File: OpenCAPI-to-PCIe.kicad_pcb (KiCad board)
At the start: 4 copper layers, 51.3 x 31.9 mm, 9 parts, among them J1 OpenCAPI_AAC_Host, J2 Conn_01x06, J3 Bus_PCI_Express_x8

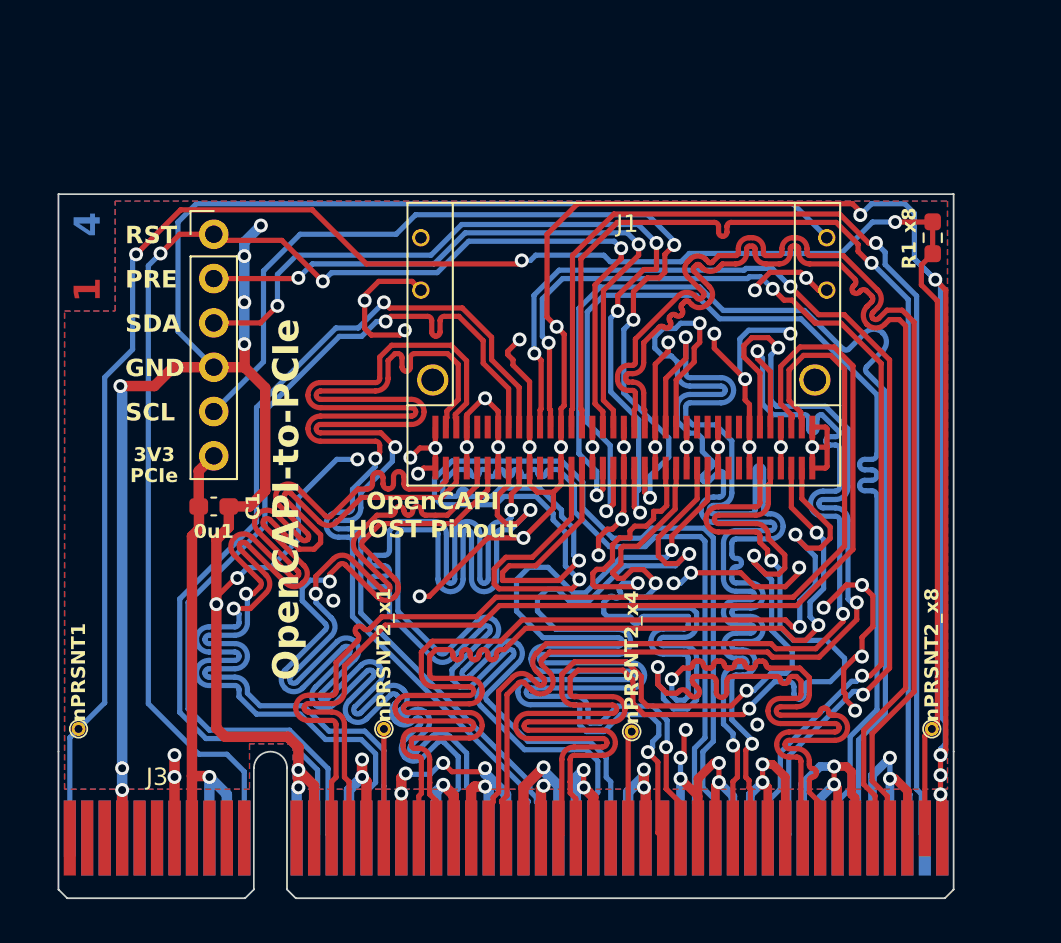
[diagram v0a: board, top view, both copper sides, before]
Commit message: Third Revision
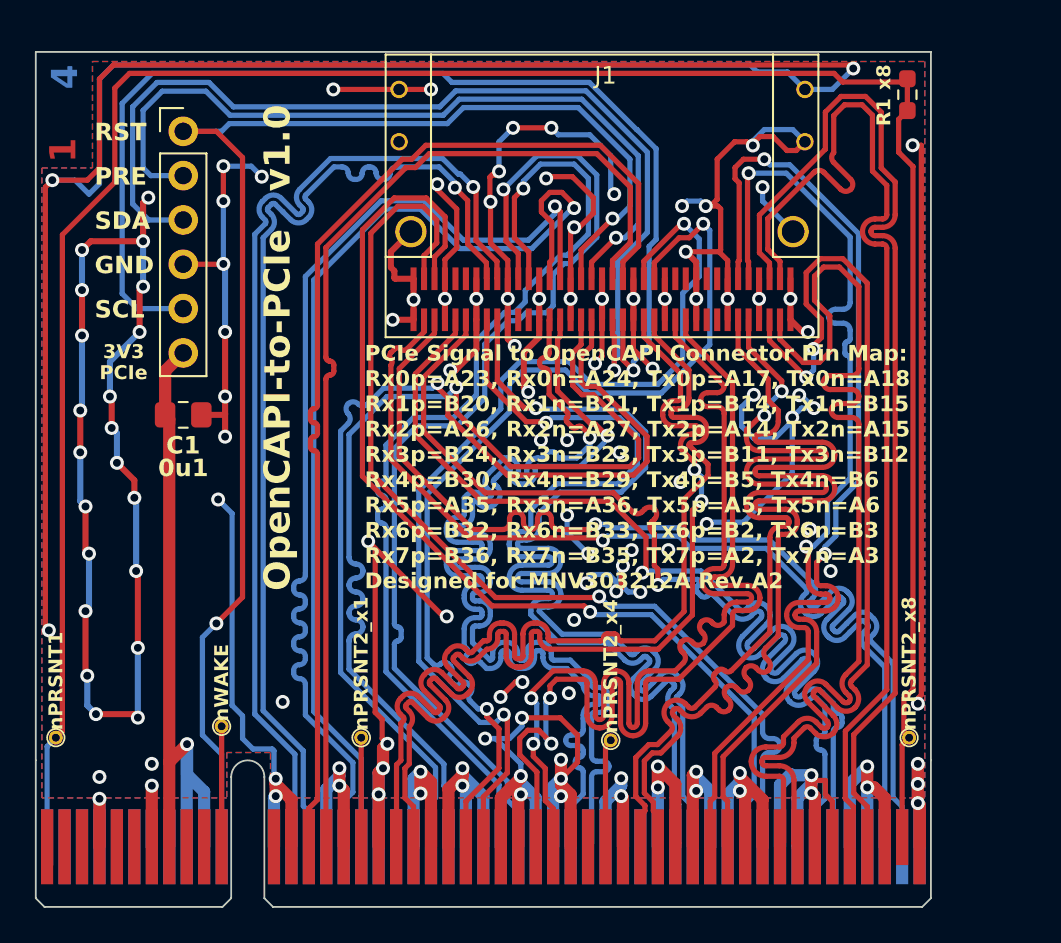
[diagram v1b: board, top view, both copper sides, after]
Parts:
- added TP4: nWAKE, TestPoint:TestPoint_THTPad_D1.0mm_Drill0.5mm, F.Cu at (60.7, 79.6)
- C1: footprint Capacitor_SMD:C_0603_1608Metric_Pad1.08x0.95mm_HandSolder -> Capacitor_SMD:C_0805_2012Metric_Pad1.18x1.45mm_HandSolder
- moved J1 8.59 mm to (71.7, 56.3)
- moved R1 8.33 mm to (100.0, 43.4)
- moved J2 6.15 mm to (58.5, 45.5)
- moved C1 5.53 mm to (58.5, 61.8)
- moved TP5 1.39 mm to (100.1, 80.2)
- moved J3 1.39 mm to (50.7, 86.5)
- moved TP1 1.39 mm to (51.2, 80.2)
- moved TP2 1.39 mm to (68.7, 80.2)
- moved TP3 1.30 mm to (83.0, 80.4)
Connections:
- J1 pad A14: Tx5_P -> Tx2_P
- J1 pad A15: Tx5_N -> Tx2_N
- J1 pad A17: Tx7_P -> Tx0_P
- J1 pad A18: Tx7_N -> Tx0_N
- J1 pad A2: Tx0_P -> Tx7_P
- J1 pad A23: Rx7_P -> Rx0_P
- J1 pad A24: Rx7_N -> Rx0_N
- J1 pad A26: Rx5_P -> Rx2_P
- J1 pad A27: Rx5_N -> Rx2_N
- J1 pad A3: Tx0_N -> Tx7_N
- J1 pad A35: Rx2_P -> Rx5_P
- J1 pad A36: Rx2_N -> Rx5_N
- J1 pad A5: Tx2_P -> Tx5_P
- J1 pad A6: Tx2_N -> Tx5_N
- J1 pad B11: Tx4_P -> Tx3_P
- J1 pad B12: Tx4_N -> Tx3_N
- J1 pad B14: Tx6_P -> Tx1_P
- J1 pad B15: Tx6_N -> Tx1_N
- J1 pad B2: Tx1_P -> Tx6_P
- J1 pad B20: Rx6_P -> Rx1_P
- J1 pad B21: Rx6_N -> Rx1_N
- J1 pad B23: Rx4_P -> Rx3_N
- J1 pad B24: Rx4_N -> Rx3_P
- J1 pad B29: Rx3_P -> Rx4_N
- J1 pad B3: Tx1_N -> Tx6_N
- J1 pad B30: Rx3_N -> Rx4_P
- J1 pad B32: Rx1_P -> Rx6_P
- J1 pad B33: Rx1_N -> Rx6_N
- J1 pad B35: Rx0_P -> Rx7_N
- J1 pad B36: Rx0_N -> Rx7_P
- J1 pad B5: Tx3_P -> Tx4_P
- J1 pad B6: Tx3_N -> Tx4_N
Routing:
- net GND: track 523.6 -> 671.4 mm, vias 83 -> 132
- net Net-(J3-~{PRSNT1}): track 119.5 -> 135.1 mm, vias 3 -> 0
- net +3.3V: track 30.9 -> 42.4 mm
- net SCL: track 54.4 -> 64.2 mm, vias 3 -> 1
- net PRE_DETECT: track 37.3 -> 45.4 mm, vias 2 -> 1
- net SDA: track 49.6 -> 57.6 mm, vias 4 -> 1
- net nWAKE: track 0.00 -> 6.90 mm
- net Rx4_N: track 65.1 -> 59.2 mm
- net Tx2_N: track 62.5 -> 57.5 mm
- net Tx3_N: track 64.4 -> 59.4 mm
- net Tx4_P: track 62.1 -> 57.1 mm
- net REFCLK_P: track 55.1 -> 59.9 mm
- net REFCLK_N: track 55.1 -> 59.8 mm
- net Rx4_P: track 63.9 -> 59.4 mm
- net Rx3_N: track 63.0 -> 58.5 mm
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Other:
- board size 51.3 x 31.9 mm -> 51.3 x 40.6 mm
- board text added: "OpenCAPI-to-PCIe v1.0"
- board text added: "PCIe Signal to OpenCAPI Connector Pin Map: Rx0p=A23, Rx0n=A24, Tx0p=A17, Tx0n=A18 Rx1p=B20, Rx1n=B21, Tx1p=B14, Tx1n=B15 Rx2p=A26, Rx2n=A27, Tx2p=A14, Tx2n=A15 Rx3p=B24, Rx3n=B23, Tx3p=B11, Tx3n=B12 Rx4p=B30, Rx4n=B29, Tx4p=B5, Tx4n=B6 Rx5p=A35, Rx5n=A36, Tx5p=A5, Tx5n=A6 Rx6p=B32, Rx6n=B33, Tx6p=B2, Tx6n=B3 Rx7p=B36, Rx7n=B35, Tx7p=A2, Tx7n=A3 Designed for MNV303212A Rev.A2"
- board text removed: "OpenCAPI HOST Pinout"
- board text removed: "OpenCAPI-to-PCIe"
